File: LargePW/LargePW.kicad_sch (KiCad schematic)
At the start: 39 parts, among them J1 Conn_01x02_Female, J10 Conn_01x02_Female, J11 Conn_01x02_Female, J12 Conn_01x02_Female, J13 Conn_01x02_Female, J2 Conn_01x02_Female, J3 Conn_01x02_Female, J4 Conn_01x02_Female, J5 Conn_01x02_Female, J6 Conn_01x02_Female, J7 Conn_01x02_Female, J8 Conn_01x02_Female, J9 Conn_01x02_Female, K1 RAYEX-L90, Q1 TJ60S04M3L, Q2 TJ60S04M3L, Q3 TJ60S04M3L, Q4 TJ60S04M3L, Q5 BSS138, SW1 SW_SPST

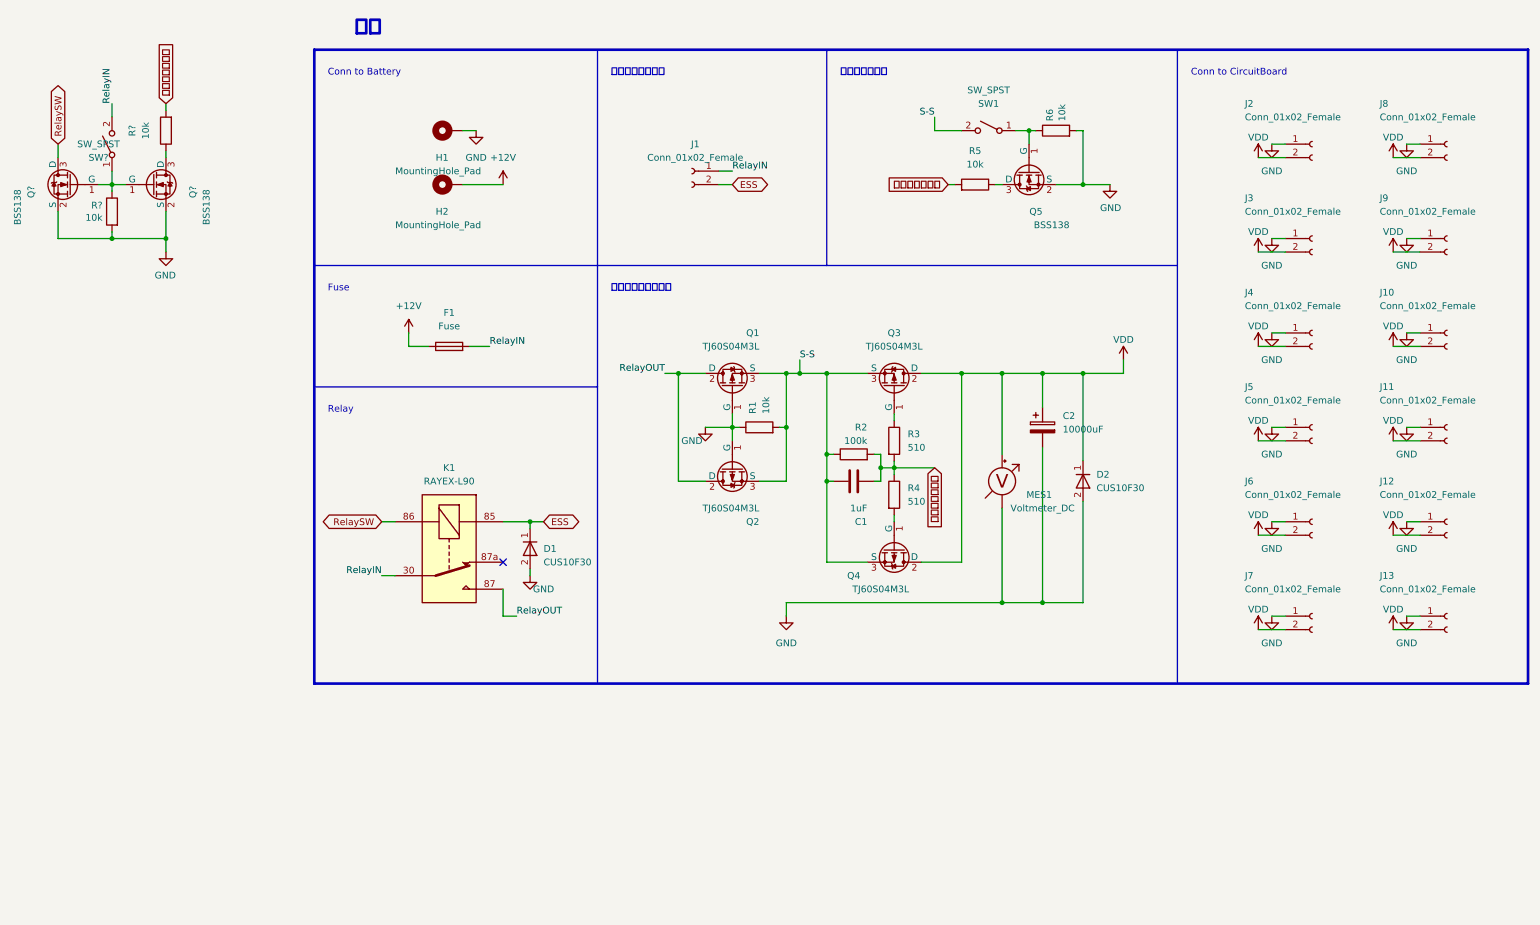
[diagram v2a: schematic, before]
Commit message: DCDC回路図変更
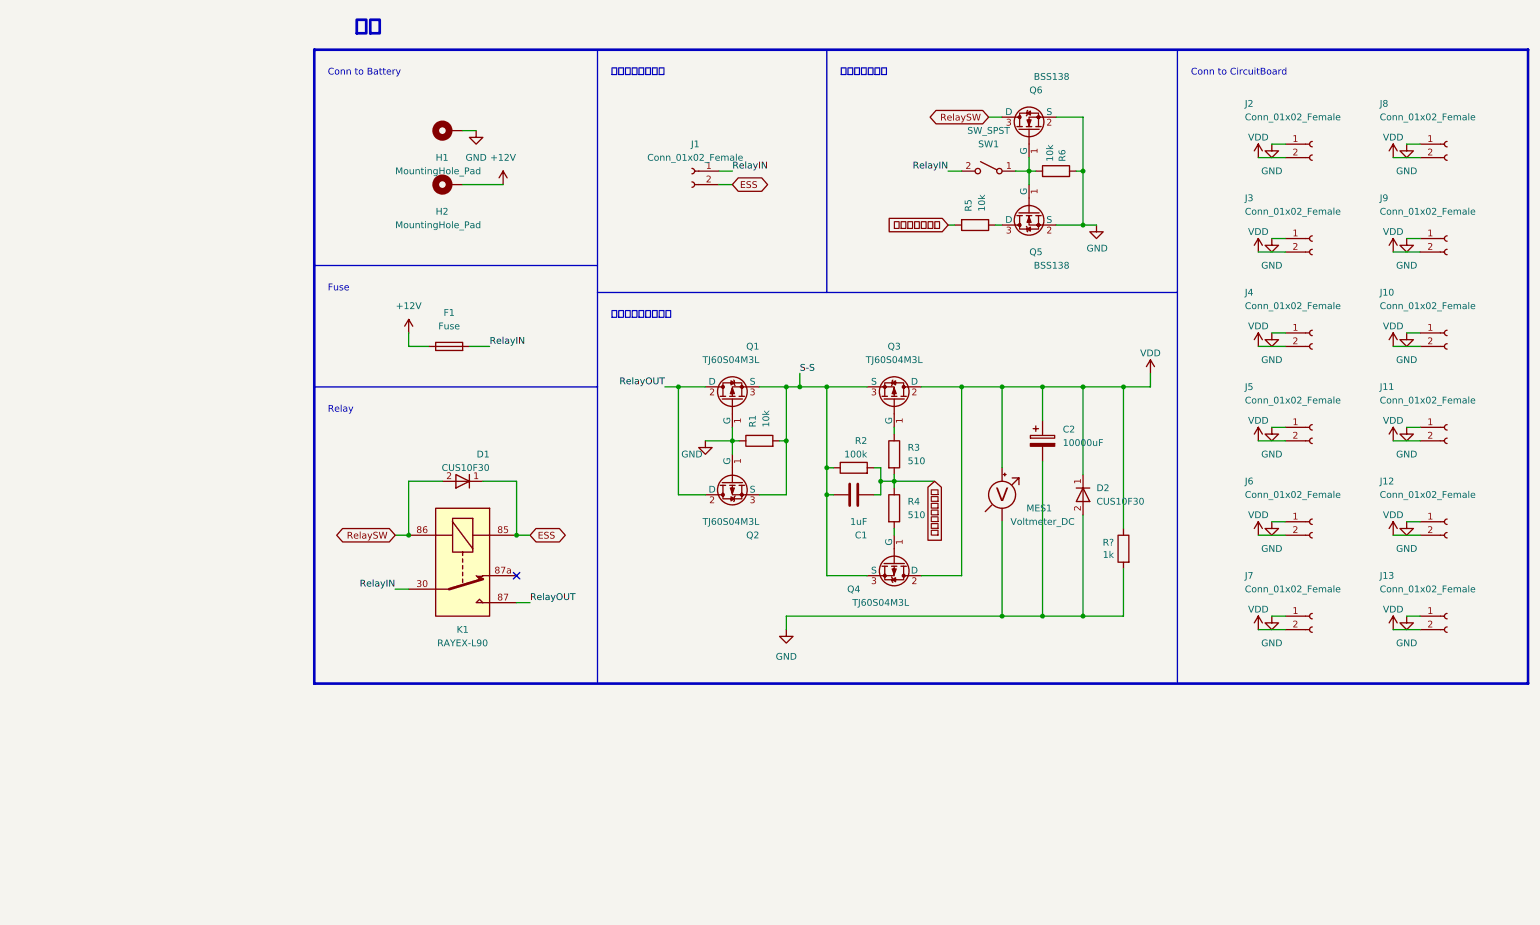
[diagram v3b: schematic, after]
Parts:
- removed Q?: BSS138, Package_TO_SOT_SMD:SOT-23_Handsoldering, symbol Device:Q_NMOS_GSD
- removed R? (x2): 10k, Resistor_SMD:R_0603_1608Metric_Pad0.98x0.95mm_HandSolder, symbol Device:R
- removed SW?: SW_SPST, Rocker_Switch:DS-850K-S-ON, symbol Switch:SW_SPST
- added R?: 1k, Resistor_SMD:R_0603_1608Metric_Pad0.98x0.95mm_HandSolder, symbol Device:R
- C1: footprint Capacitor_SMD:C_0805_2012Metric_Pad1.18x1.45mm_HandSolder -> Capacitor_SMD:C_0603_1608Metric_Pad1.08x0.95mm_HandSolder
- Q1, Q2, Q3, Q4: footprint Package_TO_SOT_SMD:TO-252-3_TabPin2 -> Package_TO_SOT_SMD:TO-252-2
- gave numbers to parts that had none: 1
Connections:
- net GND: now also R6.1, R?.2; no longer D1.2 (A), R6.2
- net RelayIN: now also SW1.2 (B)
- net RelaySW: now also D1.2 (A)
- net S-S: no longer SW1.2 (B)
- net VDD: now also R?.1
- net at Q5.1 (G), SW1.1 (A): now also Q6.1 (G), R6.2; no longer R6.1
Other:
- moved on the sheet: C1, C2, D1, D2, K1, MES1, Q1, Q2, Q3, Q4, Q5, Q6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

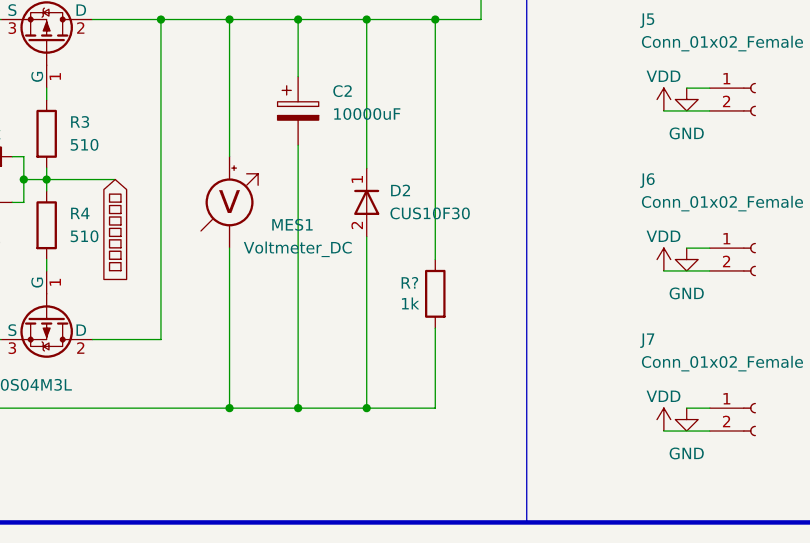
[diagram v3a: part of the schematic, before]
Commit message: 多分完成
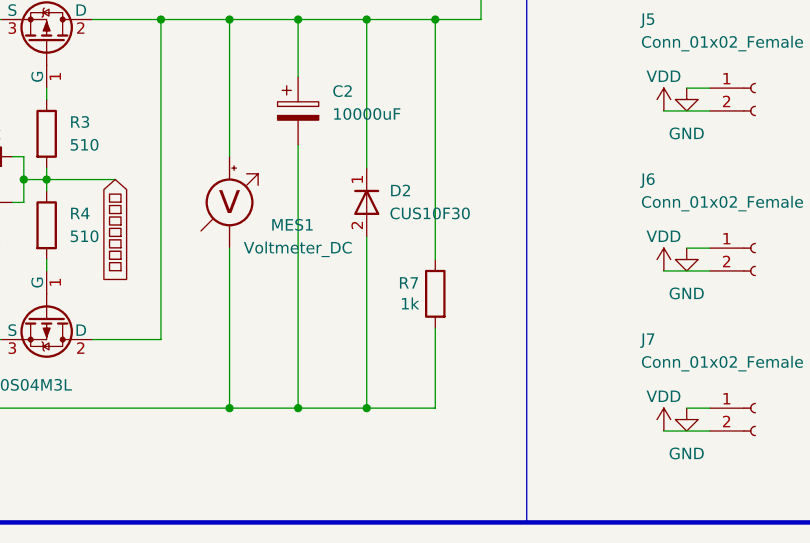
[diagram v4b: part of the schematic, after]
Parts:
- gave numbers to parts that had none: 1
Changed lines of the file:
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@@
   (symbol (lib_id "Device:R") (at 182.88 127 0) (mirror y) (unit 1)
     (in_bom yes) (on_board yes)
-    (property "Reference" "R?" (id 0) (at 181.102 125.8316 0)
+    (property "Reference" "R7" (id 0) (at 181.102 125.8316 0)
       (effects (font (size 1.27 1.27)) (justify left))
     )
@@
     )
     (path "/8bc9768e-90d7-44b5-9c64-cc5d37039949"
-      (reference "R?") (unit 1) (value "1k") (footprint "Resistor_SMD:R_0603_1608Metric_Pad0.98x0.95mm_HandSolder")
+      (reference "R7") (unit 1) (value "1k") (footprint "Resistor_SMD:R_0603_1608Metric_Pad0.98x0.95mm_HandSolder")
     )
     (path "/37affa96-b221-495c-84a8-e7d6fa125973"
